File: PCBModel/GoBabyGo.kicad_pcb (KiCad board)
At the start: 2 copper layers, 27 parts, among them J1 Conn_01x02_Pin, Q1 Q_NPN_BCE, Q2 Q_NPN_BCE, U1 NE555P, U2 NE555P

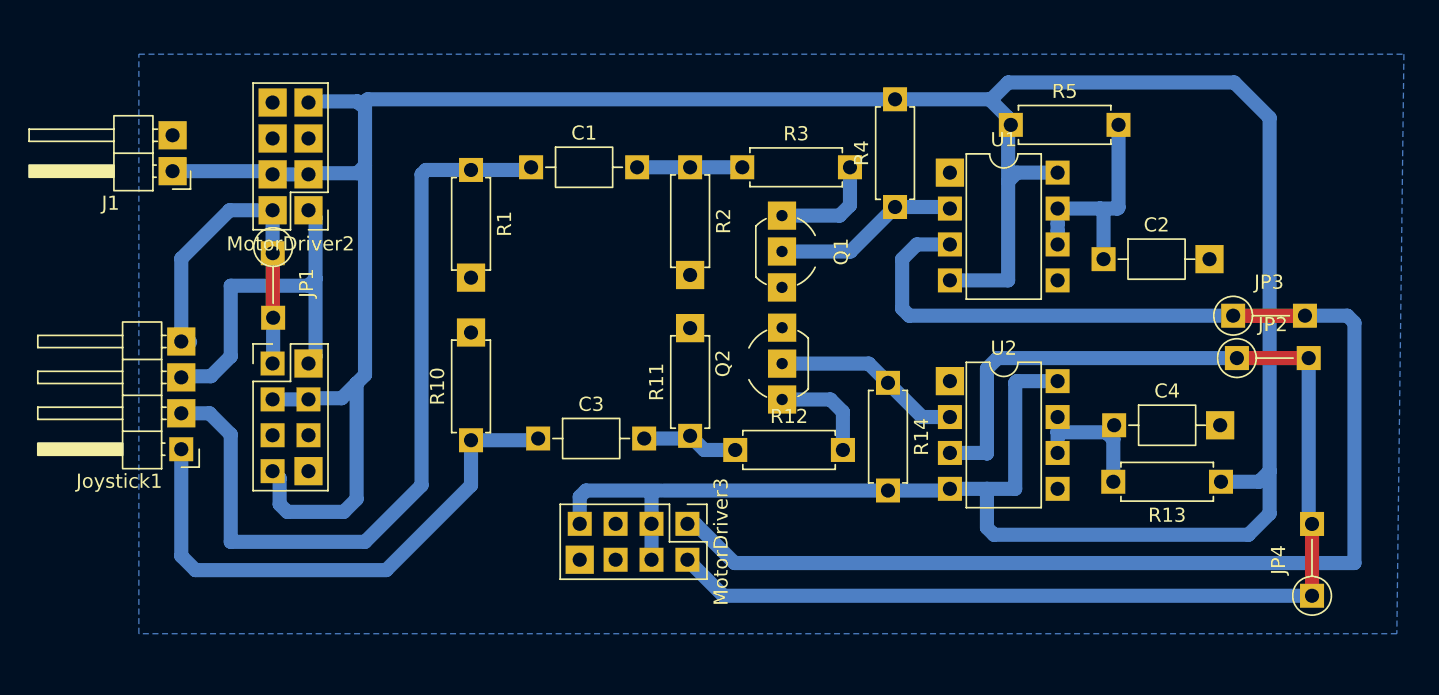
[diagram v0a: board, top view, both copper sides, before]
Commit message: PCB review.
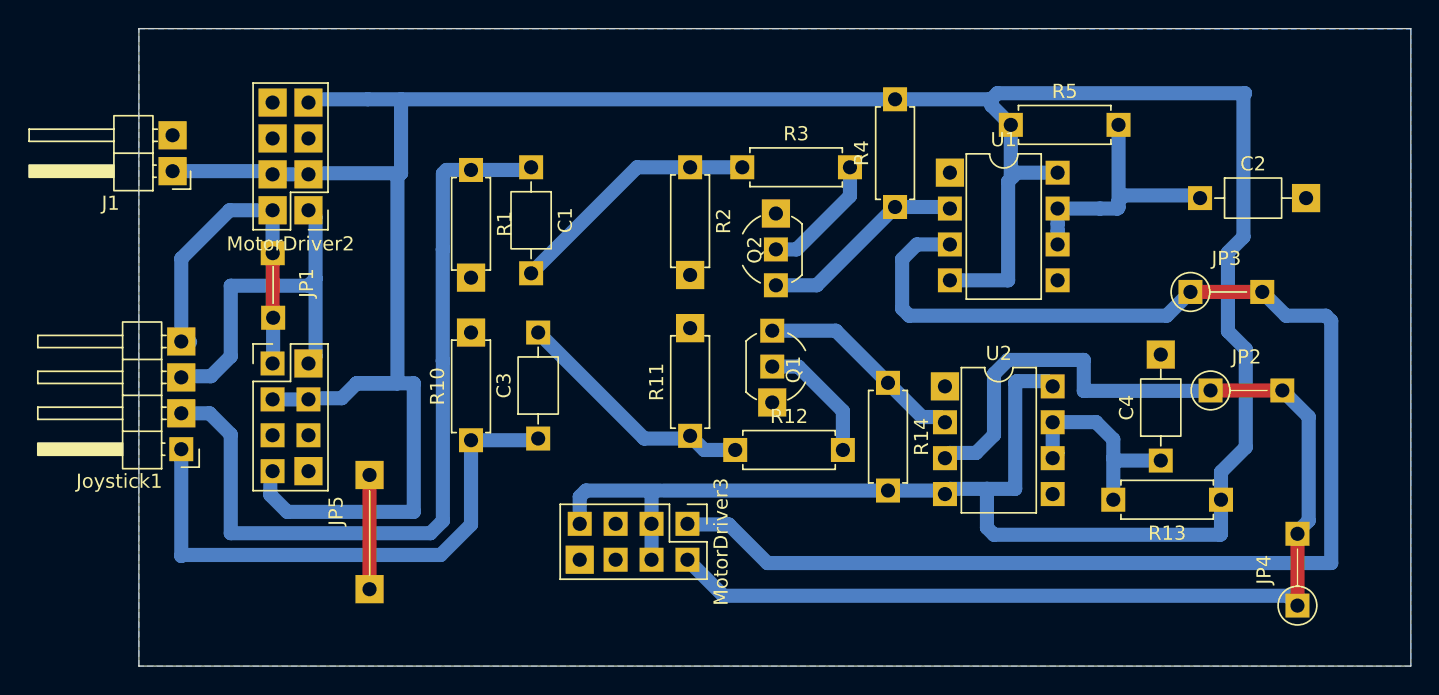
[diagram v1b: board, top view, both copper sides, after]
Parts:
- added JP5: Jumper_GND, Resistor_THT:R_Axial_DIN0207_L6.3mm_D2.5mm_P5.08mm_Vertical, F.Cu at (123.8, 109.8)
- Q1, Q2: value Q_NPN_BCE -> NPN
- moved Q1 8.17 mm to (152.3, 94.6)
- moved Q2 8.09 mm to (152.6, 91.3)
- moved C2 8.08 mm to (182.6, 85.2)
- moved C4 4.14 mm to (179.8, 103.8), turned to 90 degrees
- moved JP3 3.46 mm to (181.9, 91.8)
- moved JP2 2.95 mm to (183.3, 98.8)
- moved R13 1.27 mm to (184.1, 106.5)
- moved JP4 1.24 mm to (189.5, 114.0)
- moved U2 0.51 mm to (164.5, 98.5)
- turned C1 to -90 degrees
- turned C3 to 90 degrees
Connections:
- Q1 pad 1: Net-(Q1-B) -> Net-(Q1-C)
- Q1 pad 2: Net-(Q1-C) -> Net-(Q1-B)
- Q2 pad 1: Net-(Q2-B) -> Net-(Q2-C)
- Q2 pad 2: Net-(Q2-C) -> Net-(Q2-B)
- R12 pad 2: Net-(Q2-B) -> Net-(Q1-B)
- R14 pad 1: Net-(Q2-C) -> Net-(Q1-C)
- R3 pad 2: Net-(Q1-B) -> Net-(Q2-B)
- R4 pad 1: Net-(Q1-C) -> Net-(Q2-C)
- U1 pad 2: Net-(Q1-C) -> Net-(Q2-C)
- U2 pad 2: Net-(Q2-C) -> Net-(Q1-C)
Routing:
- net Net-(C3-Pad2): track 7.37 -> 18.0 mm
- net Net-(C1-Pad2): track 7.44 -> 18.0 mm
- net GND: track 0.00 -> 8.08 mm
- net +5V: track 251.6 -> 259.1 mm
- net Net-(U2-DISCH): track 11.0 -> 15.6 mm
- net Net-(U1-DISCH): track 16.4 -> 18.7 mm
- net Net-(Q1-C): track 13.2 -> 15.2 mm
- net /L_o: track 105.1 -> 103.2 mm
- net Net-(Q2-B): track 7.36 -> 8.84 mm
- net /R_o: track 94.2 -> 92.8 mm
- net Net-(Q1-B): track 7.80 -> 9.05 mm
- net Net-(Q2-C): track 13.4 -> 14.7 mm
- net /R: track 39.1 -> 39.9 mm
- net /L: track 56.8 -> 57.5 mm
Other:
- board outline added: 90 x 45.1 mm
